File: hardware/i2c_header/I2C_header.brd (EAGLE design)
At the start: 27 x 30.7 mm, 5 parts

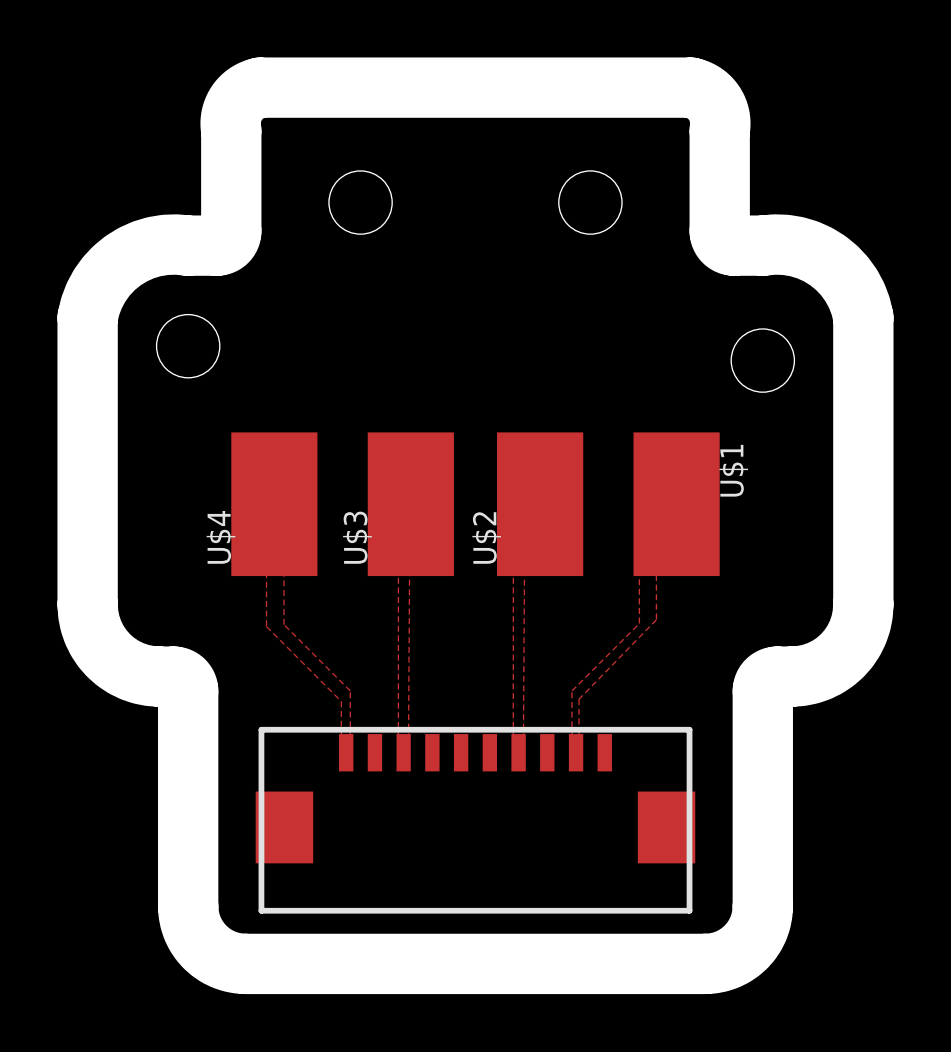
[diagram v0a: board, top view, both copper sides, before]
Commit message: Latest hardware designs
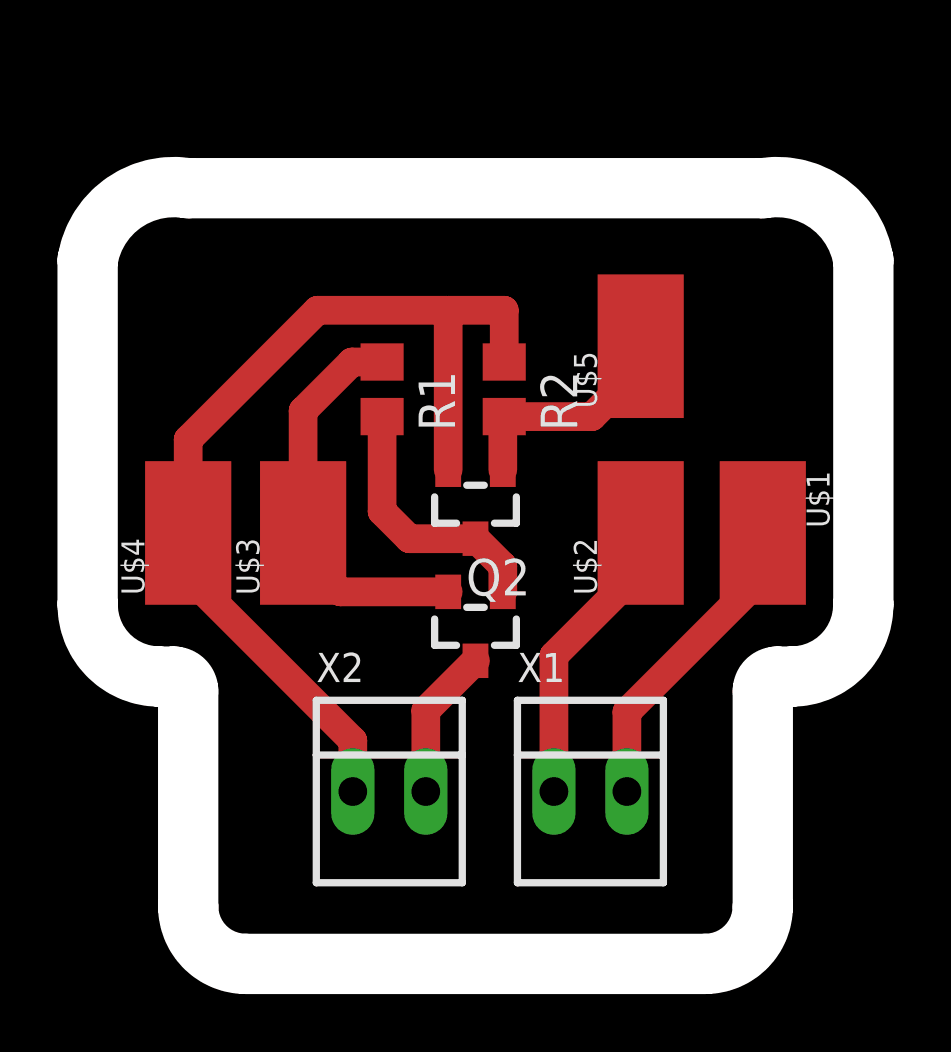
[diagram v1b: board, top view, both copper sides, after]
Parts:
- added Q1: BSS84, SIG_Parts:SOT-23-3
- added Q2: BSS138, SIG_Parts:SOT-23-3
- added R1, R2: (no value), SIG_Parts:SMD_0805
- added U$5: PAD3.0X5.0, SIG_Parts:PAD3X5
- added X1: 22-23-2021, con-molex:22-23-2021
- X2: value (none) -> 22-23-2021; device SIG_Parts:FFC_1.0X10_LARGE_PADS -> con-molex:22-23-2021
- moved U$3 3.88 mm to (4.00, 14.0)
- moved U$2 3.64 mm to (15.8, 14.0)
- moved U$1 3.16 mm to (20.0, 14.0)
- moved U$4 3.16 mm to (0.00, 14.0)
- moved X2 3.00 mm to (7.00, 5.00)
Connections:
- new net N$1: Q1.3, X2.2
- new net N$2: Q1.1, Q2.3, R1.2
- new net PWR_ON: Q2.1, R2.2, U$5.P$1
- net +3V3: now also Q1.2, R1.1; no longer X2.P$3
- net GND: now also Q2.2, R2.1, X2.1; no longer X2.P$1
- net SCL: now also X1.2; no longer X2.P$9
- net SDA: now also X1.1; no longer X2.P$7
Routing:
- net GND: track 0.00 -> 34.9 mm
- net +3V3: track 0.00 -> 14.4 mm
- net SCL: track 0.00 -> 11.0 mm
- net SDA: track 0.00 -> 10.3 mm
- net N$2: track 0.00 -> 9.19 mm
- net PWR_ON: track 0.00 -> 8.07 mm
- net N$1: track 0.00 -> 5.27 mm
- removed copper zone on layer 1, net +3V3
- removed copper zone on layer 1, net GND
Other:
- board size 27 x 30.7 mm -> 27 x 27 mm
